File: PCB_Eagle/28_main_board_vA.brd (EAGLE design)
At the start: 20 x 25 mm, 69 parts, among them SW1 SWITCH_G2SM, SW2 SWITCH_G2SM, U2 MCP1703-30, U3 STM8L051F3, U4 LIS3DH, X2 SWIM-2, Y1 32kHz

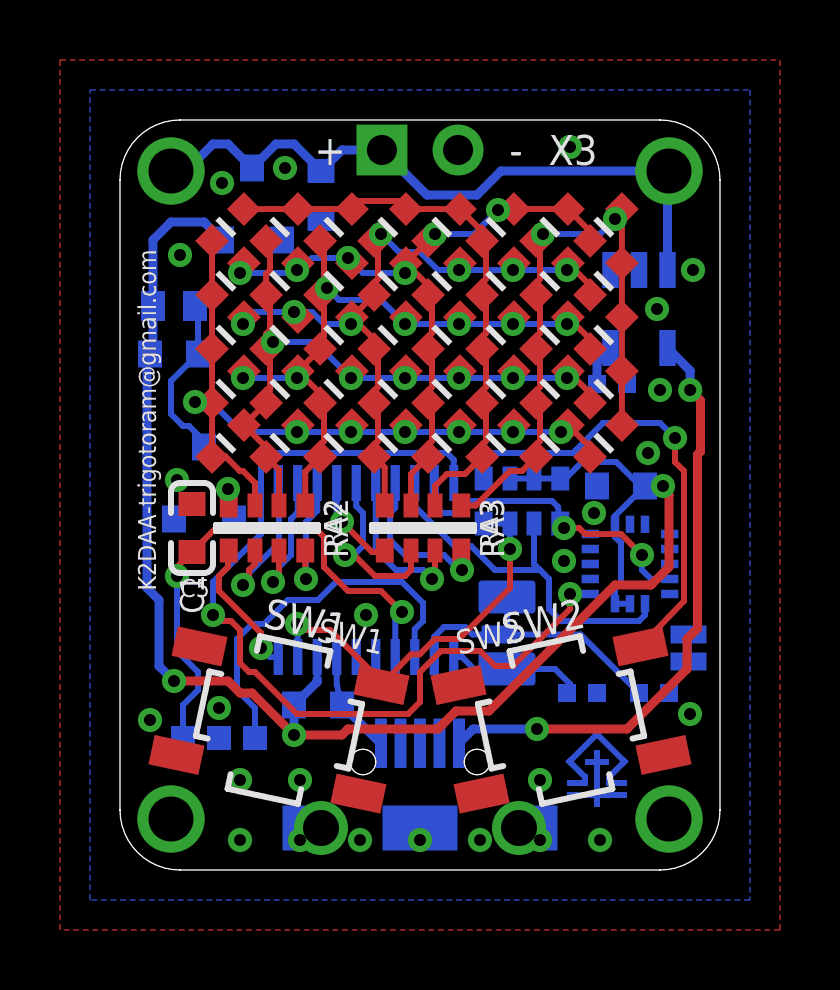
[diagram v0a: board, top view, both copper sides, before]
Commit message: v
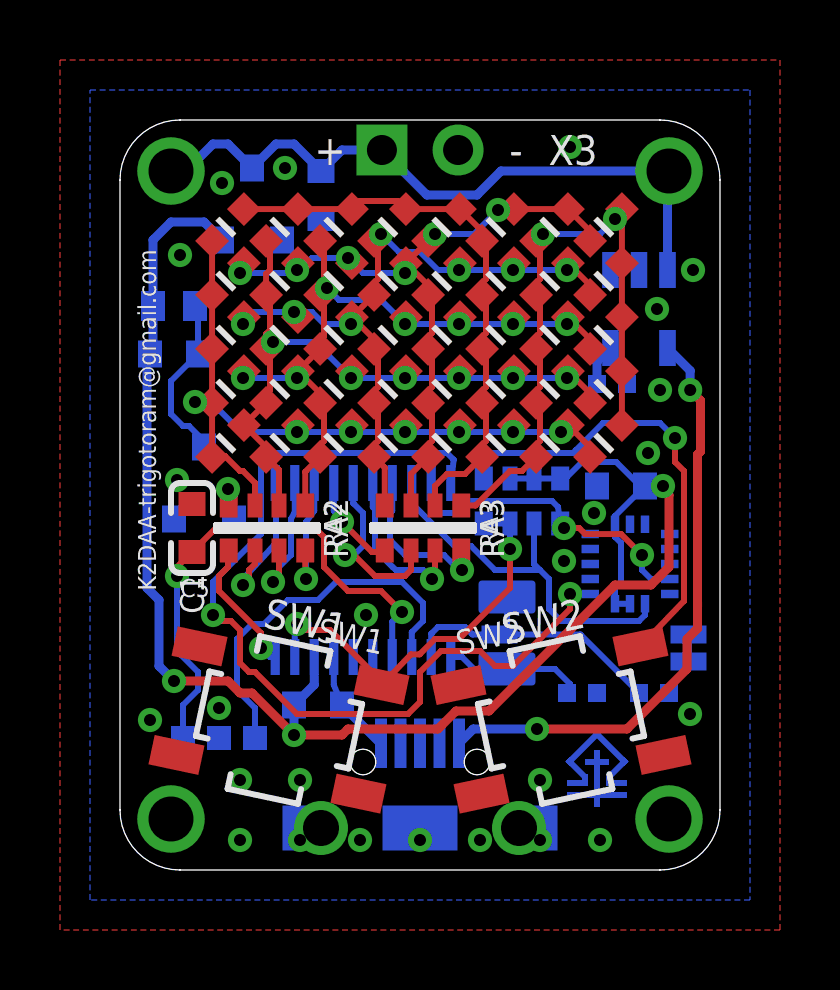
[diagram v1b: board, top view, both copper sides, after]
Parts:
- moved U3 0.10 mm to (8.10, 10.0)
